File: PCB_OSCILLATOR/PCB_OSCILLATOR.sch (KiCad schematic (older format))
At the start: 100 parts, among them J1 Jumper, J10 Jumper, J11 Jumper, J12 Jumper, J13 Jumper, J14 Jumper, J15 Jumper, J16 Jumper, J2 Jumper, J3 Jumper, J4 Jumper, J5 Jumper, J6 Jumper, J7 Jumper, J8 Jumper, J9 Jumper, P1 CONN_01X04, P2 MCLK_EXTERNAL, P3 SPI_AD5270_1, P4 SPI_AD5270_2, P5 SPI_AD9833_1, P6 SPI_AD9833_2, P7 CONN_01X04, U1 AD5270, U10 ADR291, U2 AD8421, U3 AD9833, U4 AD5270, U5 AD8421, U6 AD9833, U7 ADG819, U8 ADP3303, U9 AD8651

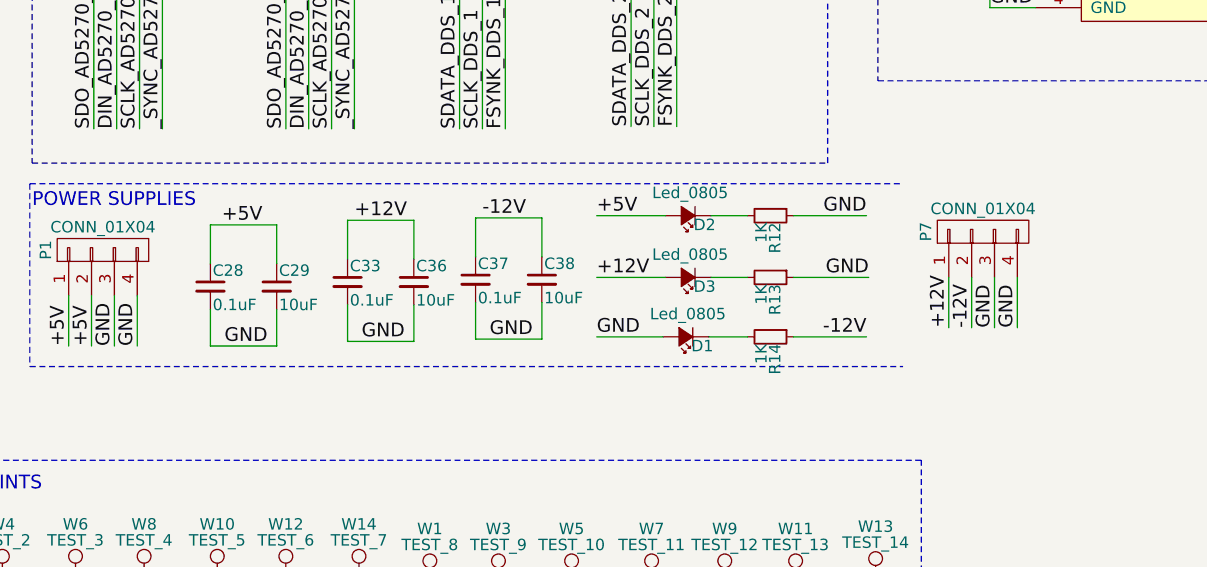
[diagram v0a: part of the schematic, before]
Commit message: PCB 95%
Terminar de hacer planos que se crean convenientes//
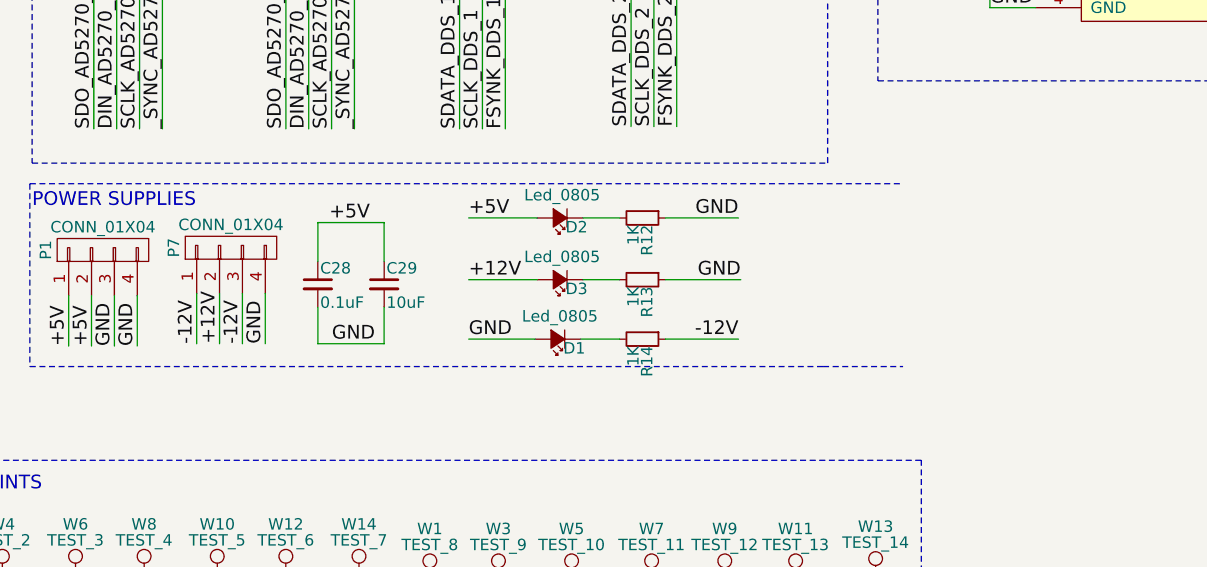
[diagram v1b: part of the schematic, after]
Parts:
- removed C33, C37: 0.1uF, Capacitors_SMD:C_0805_HandSoldering, symbol 0.1uF
- removed C36, C38: 10uF, Capacitors_SMD:C_0805_HandSoldering, symbol 10uF
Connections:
- net +12V: now also P7.2 (P2); no longer P7.1 (P1)
- net -12V: now also P7.1 (P1), P7.3 (P3); no longer P7.2 (P2)
- net GND: no longer P7.3 (P3)
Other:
- moved on the sheet: C28, C29, D1, D2, D3, P7, R12, R13, R14
